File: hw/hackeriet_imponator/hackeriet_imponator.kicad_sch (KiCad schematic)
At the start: 35 parts, among them J1 USB4085-GF-A, J2 UPDI programming, J3 External Battery Connector, J4 Shitty Add On, J5 Unused pins, SW1 SW_SPDT, SW2 User configurable, SW3 User configurable, U1 ATtiny804-SS, U2 MCP2221AxSL, U3 MPU-6050, U4 TLV70028_SOT353

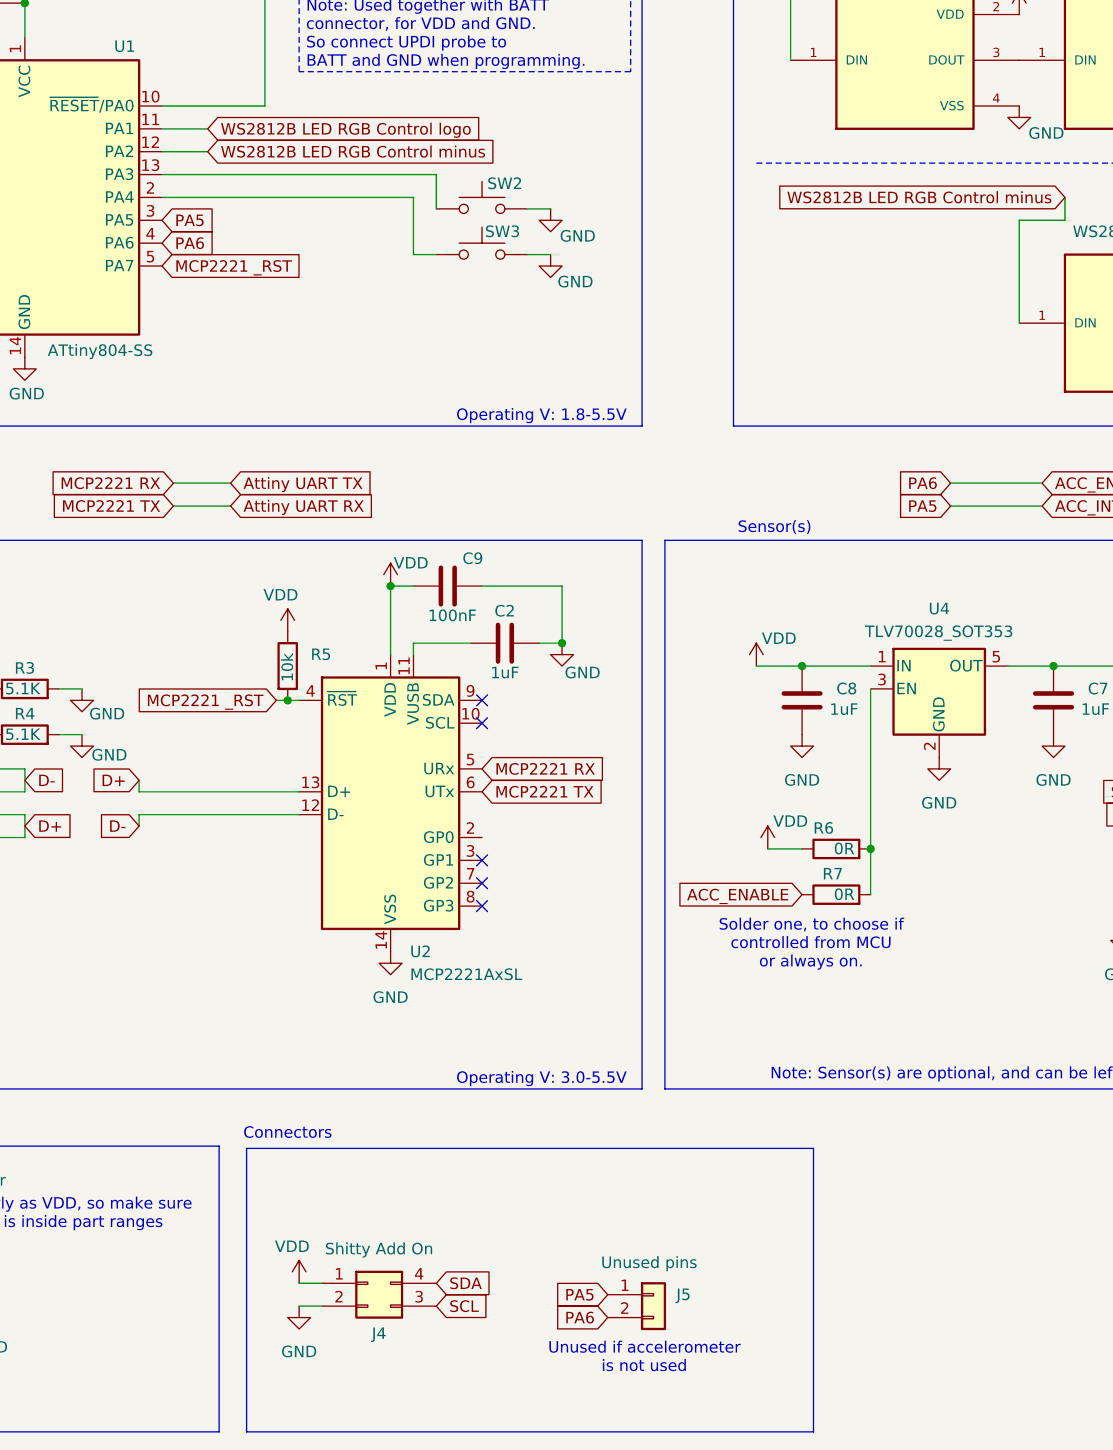
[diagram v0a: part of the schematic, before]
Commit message: More routing
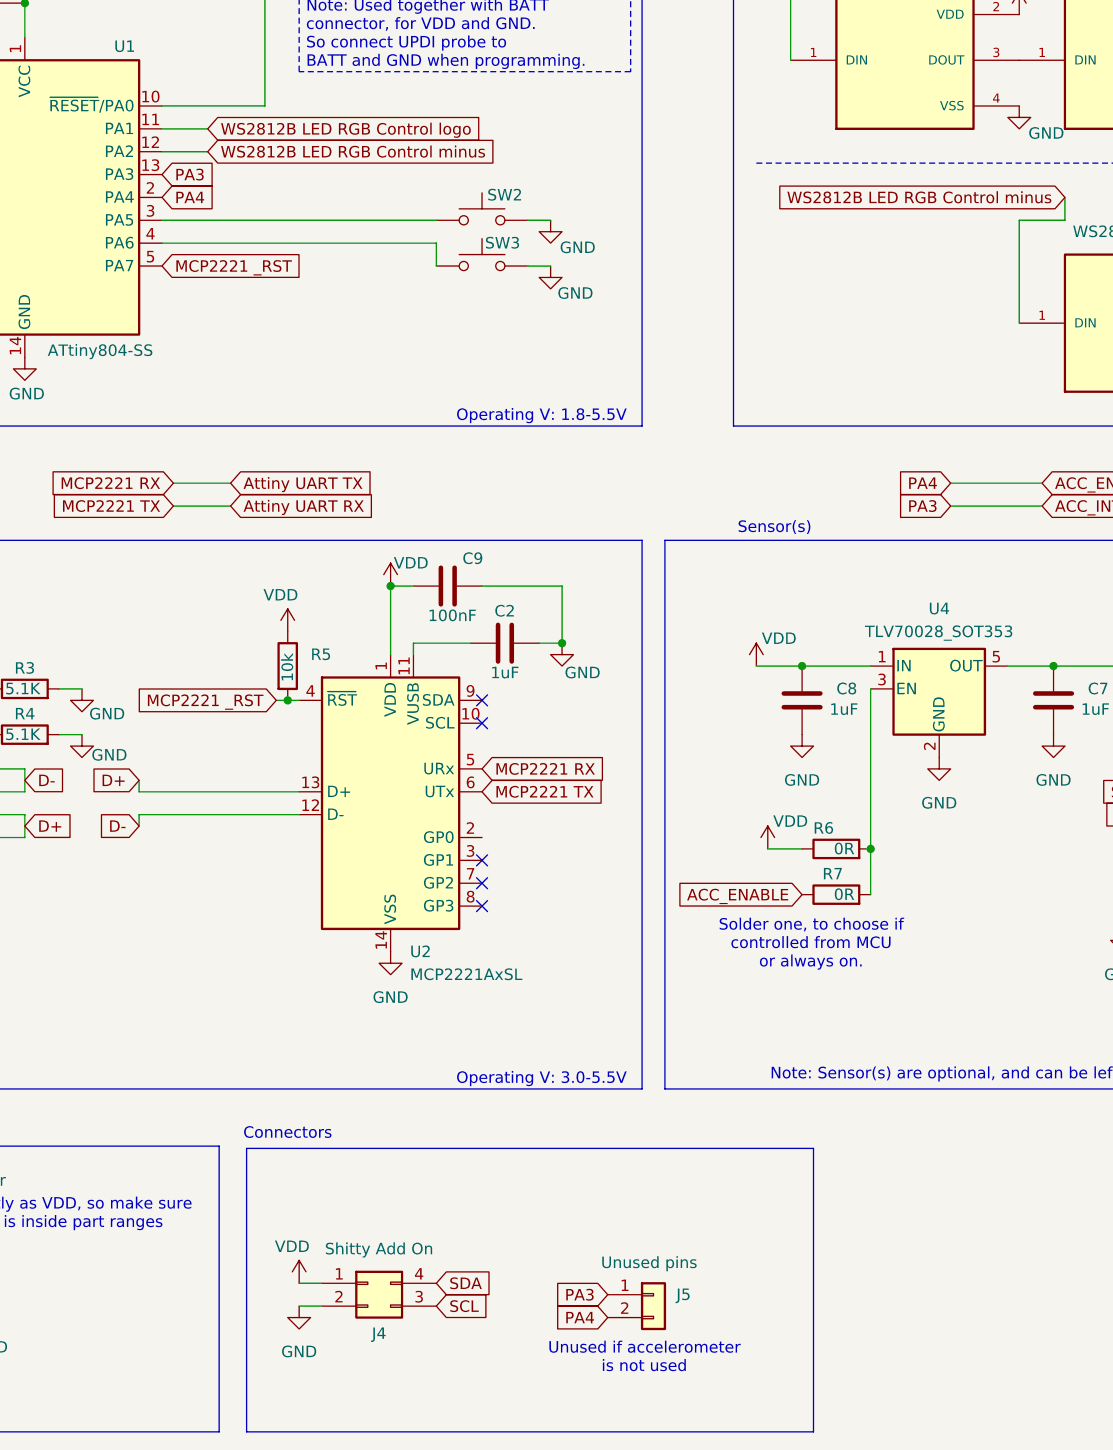
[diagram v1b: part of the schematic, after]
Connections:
- net ACC_ENABLE: now also U1.2 (PA4); no longer U1.4 (PA6)
- net ACC_INT: now also U1.13 (PA3); no longer U1.3 (PA5)
- net at SW3.1: now also U1.4 (PA6); no longer U1.2 (PA4)
- net at SW2.1: now also U1.3 (PA5); no longer U1.13 (PA3)
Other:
- moved on the sheet: SW2, SW3
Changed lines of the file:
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@@
 	(wire
 		(pts
-			(xy 81.28 58.42) (xy 109.22 58.42)
+			(xy 40.64 48.26) (xy 50.8 48.26)
 		)
 		(stroke
@@
 	(wire
 		(pts
-			(xy 40.64 48.26) (xy 50.8 48.26)
+			(xy 187.96 139.7) (xy 187.96 137.16)
 		)
 		(stroke
@@
 	(wire
 		(pts
-			(xy 187.96 139.7) (xy 187.96 137.16)
+			(xy 111.76 66.04) (xy 111.76 63.5)
 		)
 		(stroke
@@
 	(wire
 		(pts
-			(xy 111.76 55.88) (xy 111.76 59.69)
+			(xy 81.28 63.5) (xy 111.76 63.5)
 		)
 		(stroke
@@
 	(wire
 		(pts
-			(xy 121.92 64.77) (xy 124.46 64.77)
+			(xy 121.92 66.04) (xy 124.46 66.04)
 		)
 		(stroke
@@
 	(wire
 		(pts
-			(xy 109.22 58.42) (xy 109.22 64.77)
+			(xy 168.91 90.17) (xy 179.07 90.17)
 		)
 		(stroke
@@
 	(wire
 		(pts
-			(xy 168.91 90.17) (xy 179.07 90.17)
+			(xy 69.85 118.11) (xy 72.39 118.11)
 		)
 		(stroke
@@
 	(wire
 		(pts
-			(xy 69.85 118.11) (xy 72.39 118.11)
+			(xy 81.28 60.96) (xy 111.76 60.96)
 		)
 		(stroke
@@
 	(wire
 		(pts
-			(xy 121.92 59.69) (xy 124.46 59.69)
+			(xy 121.92 60.96) (xy 124.46 60.96)
 		)
 		(stroke
@@
 	(wire
 		(pts
-			(xy 81.28 55.88) (xy 111.76 55.88)
-		)
-		(stroke
-			(width 0)
-			(type default)
-		)
-	)
-	(wire
-		(pts
 			(xy 62.23 114.3) (xy 62.23 113.03)
 		)
@@
 	(wire
 		(pts
-			(xy 109.22 64.77) (xy 111.76 64.77)
-		)
-		(stroke
-			(width 0)
-			(type default)
-		)
-	)
-	(wire
-		(pts
 			(xy 96.52 179.07) (xy 99.06 179.07)
 		)
@@
 		)
 	)
-	(global_label "PA5"
-		(shape input)
-		(at 81.28 60.96 0)
-		(fields_autoplaced yes)
-		(effects
-			(font
-				(size 1.27 1.27)
-			)
-			(justify left)
-		)
-		(property "Intersheetrefs" "${INTERSHEET_REFS}"
-			(at 87.8333 60.96 0)
-			(effects
-				(font
-					(size 1.27 1.27)
-				)
-				(justify left)
-				(hide yes)
-			)
-		)
-	)
 	(global_label "WS2812B LED RGB Control logo"
 		(shape input)
@@
 		)
 	)
-	(global_label "PA5"
+	(global_label "PA3"
 		(shape input)
 		(at 168.91 92.71 180)
@@
 		)
 	)
-	(global_label "PA5"
+	(global_label "PA3"
 		(shape input)
 		(at 130.81 180.34 180)
@@
 		)
 	)
-	(global_label "PA6"
+	(global_label "PA4"
 		(shape input)
 		(at 130.81 182.88 180)
@@
 		)
 	)
-	(global_label "SDA"
+	(global_label "PA4"
 		(shape input)
-		(at 111.76 179.07 0)
+		(at 81.28 58.42 0)
 		(fields_autoplaced yes)
 		(effects
@@
 		)
 		(property "Intersheetrefs" "${INTERSHEET_REFS}"
-			(at 118.3133 179.07 0)
+			(at 87.8333 58.42 0)
 			(effects
 				(font
@@
 		)
 	)
-	(global_label "D-"
+	(global_label "SDA"
 		(shape input)
-		(at 78.74 128.27 180)
+		(at 111.76 179.07 0)
 		(fields_autoplaced yes)
 		(effects
@@
 				(size 1.27 1.27)
 			)
-			(justify right)
+			(justify left)
 		)
 		(property "Intersheetrefs" "${INTERSHEET_REFS}"
-			(at 72.9124 128.27 0)
+			(at 118.3133 179.07 0)
 			(effects
 				(font
 					(size 1.27 1.27)
 				)
-				(justify right)
+				(justify left)
 				(hide yes)
 			)
 		)
 	)
-	(global_label "PA6"
+	(global_label "D-"
 		(shape input)
-		(at 81.28 63.5 0)
+		(at 78.74 128.27 180)
 		(fields_autoplaced yes)
 		(effects
@@
 				(size 1.27 1.27)
 			)
-			(justify left)
+			(justify right)
 		)
 		(property "Intersheetrefs" "${INTERSHEET_REFS}"
-			(at 87.8333 63.5 0)
+			(at 72.9124 128.27 0)
 			(effects
 				(font
 					(size 1.27 1.27)
 				)
-				(justify left)
+				(justify right)
 				(hide yes)
 			)
@@
 		)
 	)
+	(global_label "PA3"
+		(shape input)
+		(at 81.28 55.88 0)
+		(fields_autoplaced yes)
+		(effects
+			(font
+				(size 1.27 1.27)
+			)
+			(justify left)
+		)
+		(property "Intersheetrefs" "${INTERSHEET_REFS}"
+			(at 87.8333 55.88 0)
+			(effects
+				(font
+					(size 1.27 1.27)
+				)
+				(justify left)
+				(hide yes)
+			)
+		)
+	)
 	(global_label "Attiny UART RX"
 		(shape input)
@@
 		)
 	)
-	(global_label "PA6"
+	(global_label "PA4"
 		(shape input)
 		(at 168.91 90.17 180)
@@
 	(symbol
 		(lib_id "power:GND")
-		(at 124.46 59.69 0)
+		(at 124.46 60.96 0)
 		(unit 1)
 		(exclude_from_sim no)
@@
 		(dnp no)
 		(property "Reference" "#PWR038"
-			(at 124.46 66.04 0)
+			(at 124.46 67.31 0)
 			(effects
 				(font
@@
 		)
 		(property "Value" "GND"
-			(at 125.476 62.738 0)
+			(at 125.476 64.008 0)
 			(effects
 				(font
@@
 		)
 		(property "Footprint" ""
-			(at 124.46 59.69 0)
+			(at 124.46 60.96 0)
 			(effects
 				(font
@@
 		)
 		(property "Datasheet" ""
-			(at 124.46 59.69 0)
+			(at 124.46 60.96 0)
 			(effects
 				(font
@@
 		)
 		(property "Description" "Power symbol creates a global label with name \"GND\" , ground"
-			(at 124.46 59.69 0)
+			(at 124.46 60.96 0)
 			(effects
 				(font
@@
 	(symbol
 		(lib_id "Switch:SW_Push")
-		(at 116.84 64.77 0)
+		(at 116.84 66.04 0)
 		(unit 1)
 		(exclude_from_sim no)
@@
 		(dnp no)
 		(property "Reference" "SW3"
-			(at 119.126 62.23 0)
+			(at 119.126 63.5 0)
 			(effects
 				(font
@@
 		)
 		(property "Value" "User configurable"
-			(at 107.442 62.23 0)
+			(at 107.442 63.5 0)
 			(effects
 				(font
@@
 		)
 		(property "Footprint" "Button_Switch_SMD:SW_SPST_EVQP7C"
-			(at 116.84 59.69 0)
+			(at 116.84 60.96 0)
 			(effects
 				(font
@@
 		)
 		(property "Datasheet" "~"
-			(at 116.84 59.69 0)
+			(at 116.84 60.96 0)
 			(effects
 				(font
@@
 		)
 		(property "Description" "Push button switch, generic, two pins"
-			(at 116.84 64.77 0)
+			(at 116.84 66.04 0)
 			(effects
 				(font
@@
 	(symbol
 		(lib_id "Switch:SW_Push")
-		(at 116.84 59.69 0)
+		(at 116.84 60.96 0)
 		(unit 1)
 		(exclude_from_sim no)
@@
 		(dnp no)
 		(property "Reference" "SW2"
-			(at 119.38 56.896 0)
+			(at 119.38 58.166 0)
 			(effects
 				(font
@@
 		)
 		(property "Value" "User configurable"
-			(at 128.016 57.658 0)
+			(at 128.016 58.928 0)
 			(effects
 				(font
@@
 		)
 		(property "Footprint" "Button_Switch_SMD:SW_SPST_EVQP7C"
-			(at 116.84 54.61 0)
+			(at 116.84 55.88 0)
 			(effects
 				(font
@@
 		)
 		(property "Datasheet" "~"
-			(at 116.84 54.61 0)
+			(at 116.84 55.88 0)
 			(effects
 				(font
@@
 		)
 		(property "Description" "Push button switch, generic, two pins"
-			(at 116.84 59.69 0)
+			(at 116.84 60.96 0)
 			(effects
 				(font
@@
 	(symbol
 		(lib_id "power:GND")
-		(at 124.46 64.77 0)
+		(at 124.46 66.04 0)
 		(unit 1)
 		(exclude_from_sim no)
@@
 		(dnp no)
 		(property "Reference" "#PWR039"
-			(at 124.46 71.12 0)
+			(at 124.46 72.39 0)
 			(effects
 				(font
@@
 		)
 		(property "Value" "GND"
-			(at 125.222 67.818 0)
+			(at 125.222 69.088 0)
 			(effects
 				(font
@@
 		)
 		(property "Footprint" ""
-			(at 124.46 64.77 0)
+			(at 124.46 66.04 0)
 			(effects
 				(font
@@
 		)
 		(property "Datasheet" ""
-			(at 124.46 64.77 0)
+			(at 124.46 66.04 0)
 			(effects
 				(font
@@
 		)
 		(property "Description" "Power symbol creates a global label with name \"GND\" , ground"
-			(at 124.46 64.77 0)
+			(at 124.46 66.04 0)
 			(effects
 				(font
